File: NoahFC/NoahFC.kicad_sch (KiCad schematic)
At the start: 25 parts, among them J1 CH1, J10 GND, J2 CH2, J3 MPU6050, J4 FTDI, J5 VCC, J6 CH3, J7 PPM, J8 GPS, J9 CH4, U1 ATmega328-A, U3 AMS1117-5.0, Y1 16Mhz

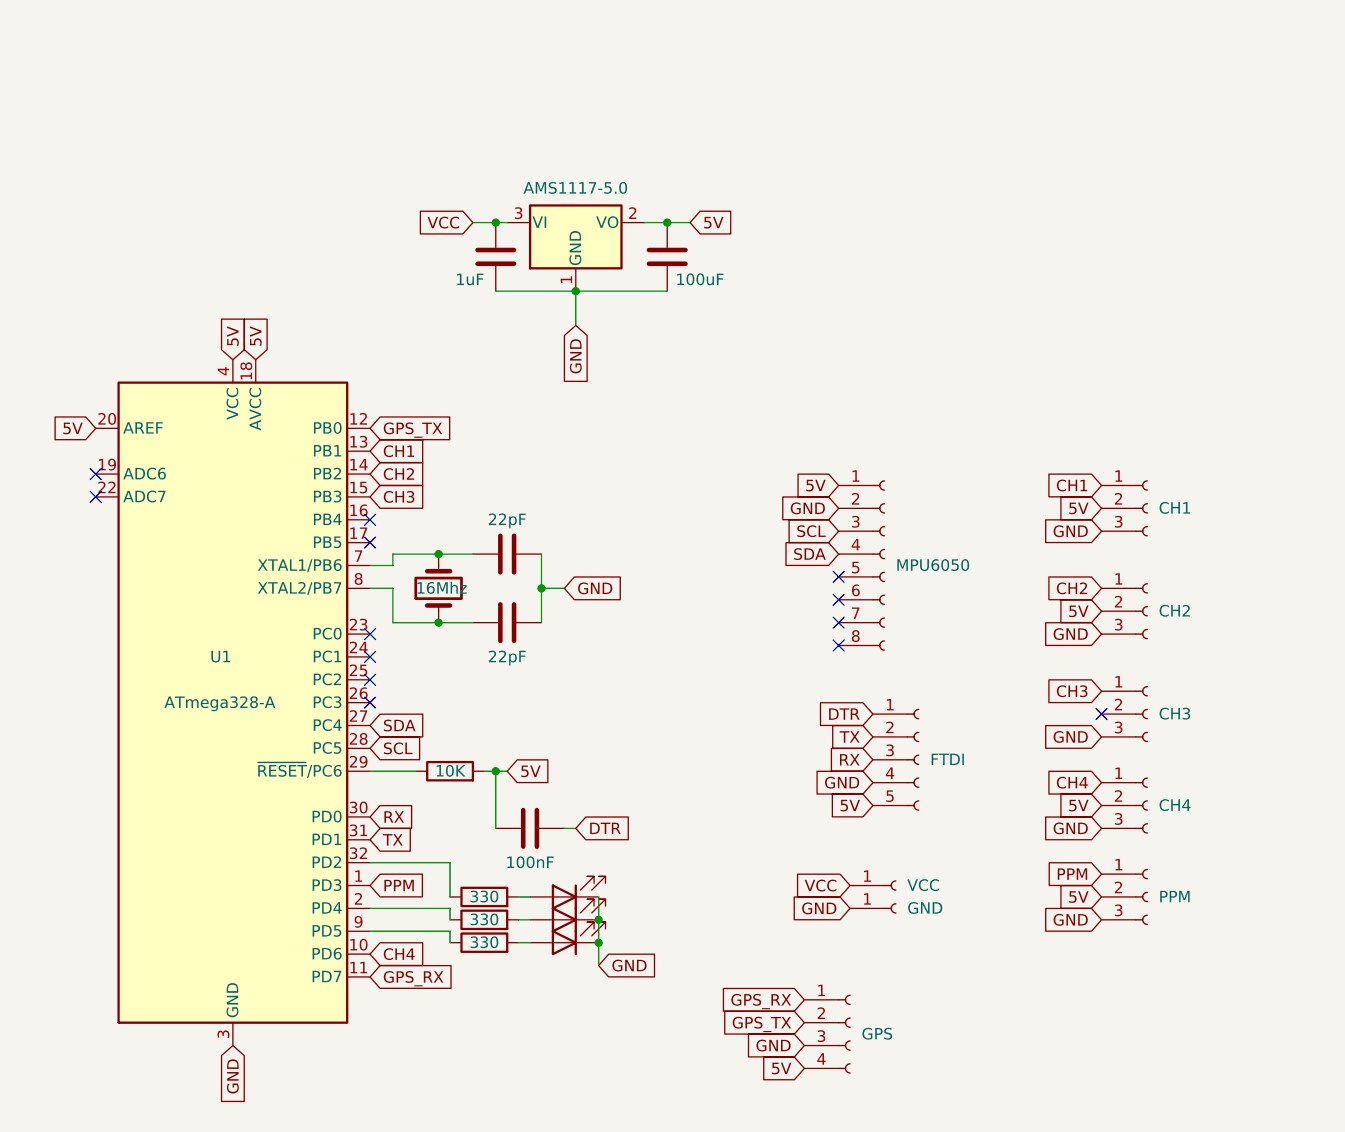
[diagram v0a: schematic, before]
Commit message: revision 1
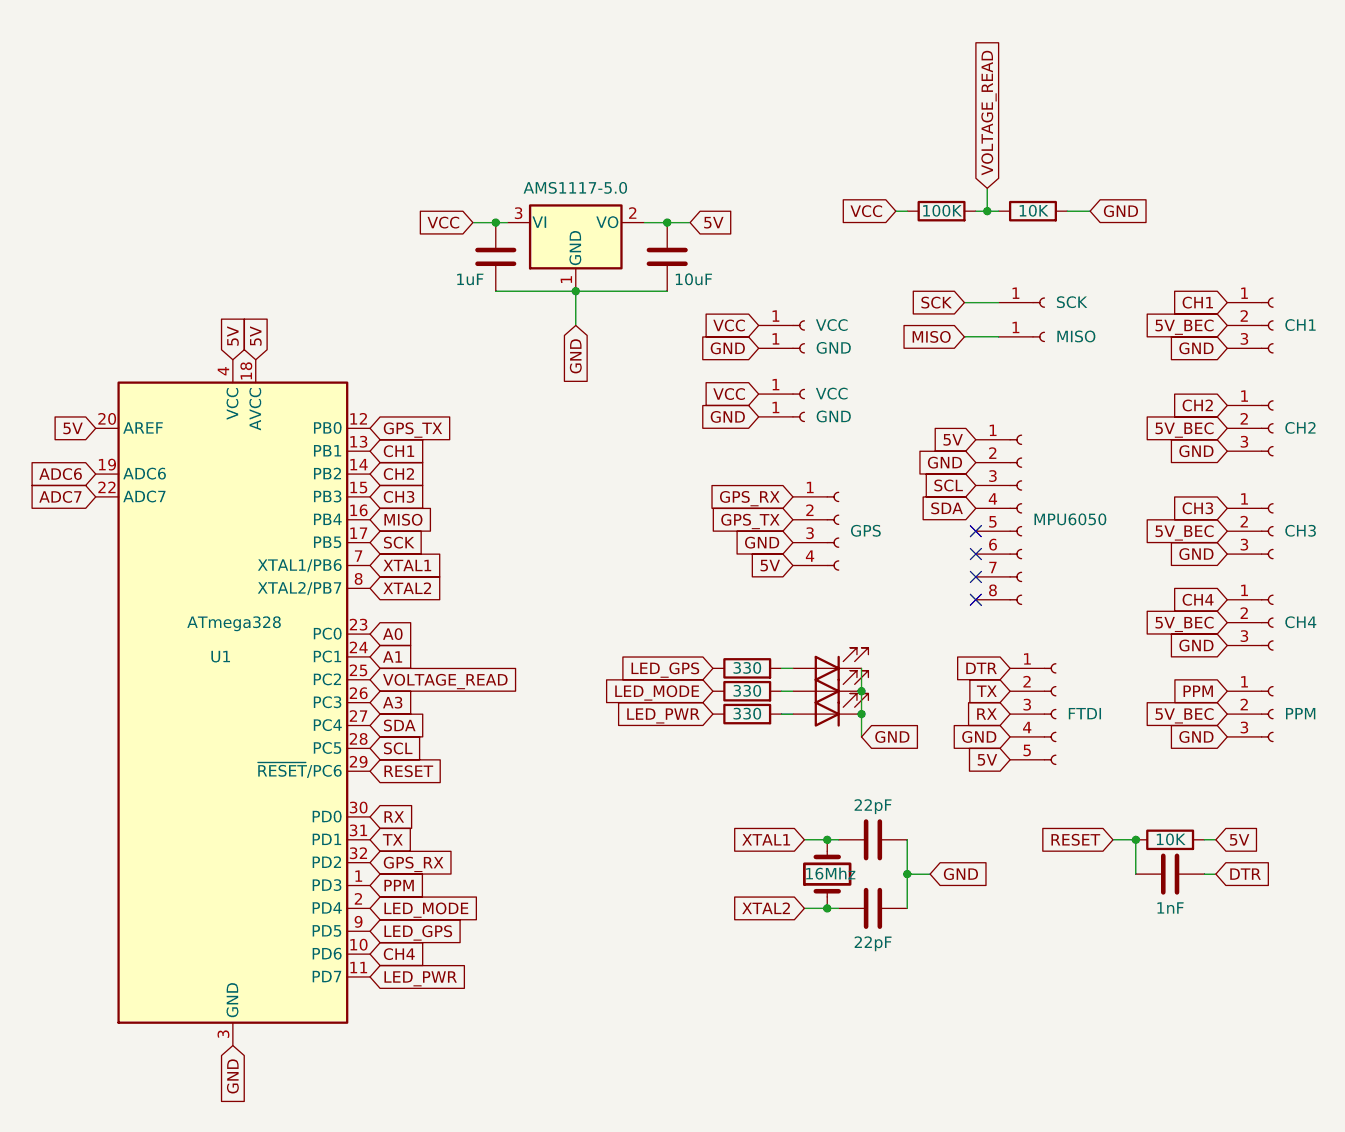
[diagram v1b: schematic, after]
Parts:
- added J11: SCK, TestPoint:TestPoint_Pad_1.0x1.0mm, symbol Connector:Conn_01x01_Female
- added J12: MISO, TestPoint:TestPoint_Pad_1.0x1.0mm, symbol Connector:Conn_01x01_Female
- added J13: VCC, TestPoint:TestPoint_Pad_4.0x4.0mm, symbol Connector:Conn_01x01_Female
- added J14: GND, TestPoint:TestPoint_Pad_4.0x4.0mm, symbol Connector:Conn_01x01_Female
- added R5: 100K, Resistor_SMD:R_0805_2012Metric, symbol Device:R
- added R6: 10K, Resistor_SMD:R_0805_2012Metric, symbol Device:R
- C3: value 100nF -> 1nF
- C5: value 100uF -> 10uF
- D1: value PWR -> GPS; footprint LED_SMD:LED_0603_1608Metric -> LED_SMD:LED_0805_2012Metric
- D2: value GPS -> MODE; footprint LED_SMD:LED_0603_1608Metric -> LED_SMD:LED_0805_2012Metric
- D3: value MODE -> PWR; footprint LED_SMD:LED_0603_1608Metric -> LED_SMD:LED_0805_2012Metric
- U1: value ATmega328-A -> ATmega328
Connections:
- net 5V: no longer C3.1, J1.2 (Pin_2), J2.2 (Pin_2), J7.2 (Pin_2), J9.2 (Pin_2)
- net GND: now also J14.1 (Pin_1), R6.2
- net GPS_RX: now also U1.32 (PD2); no longer U1.11 (PD7)
- net VCC: now also J13.1 (Pin_1), R5.1
- net XTAL1: now reaches C1.1, U1.7 (XTAL1/PB6), Y1.2
- net LED_GPS: now reaches R2.1
- net LED_GPS: now also U1.9 (PD5); no longer U1.32 (PD2)
- net MISO: now reaches U1.16 (PB4)
- net MISO: now also J12.1 (Pin_1)
- net SCK: now reaches U1.17 (PB5)
- net SCK: now also J11.1 (Pin_1)
- net ADC6: now reaches U1.19 (ADC6)
- net LED_MODE: now reaches R3.1, U1.2 (PD4)
- net ADC7: now reaches U1.22 (ADC7)
- net A0: now reaches U1.23 (PC0)
- net A1: now reaches U1.24 (PC1)
- net VOLTAGE_READ: now reaches U1.25 (PC2)
- net VOLTAGE_READ: now also R5.2, R6.1
- net A3: now reaches U1.26 (PC3)
- net RESET: now reaches R1.1, U1.29 (~{RESET}/PC6)
- net RESET: now also C3.1
- net XTAL2: now reaches C2.1, U1.8 (XTAL2/PB7), Y1.1
- net LED_PWR: now reaches R4.1
- net LED_PWR: now also U1.11 (PD7); no longer U1.9 (PD5)
- net 5V_BEC: now reaches J6.2 (Pin_2)
- net 5V_BEC: now also J1.2 (Pin_2), J2.2 (Pin_2), J7.2 (Pin_2), J9.2 (Pin_2)
- no-connect marks 13 -> 4
